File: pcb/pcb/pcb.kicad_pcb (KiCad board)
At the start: 2 copper layers, 40 x 47 mm, 8 parts, among them SW1 SW_SPDT, U1 Pimoroni_LiPo_Amigo, U2 Timecube_Accelerometer, U3 Tiny2040, U5 E-ink_Driver

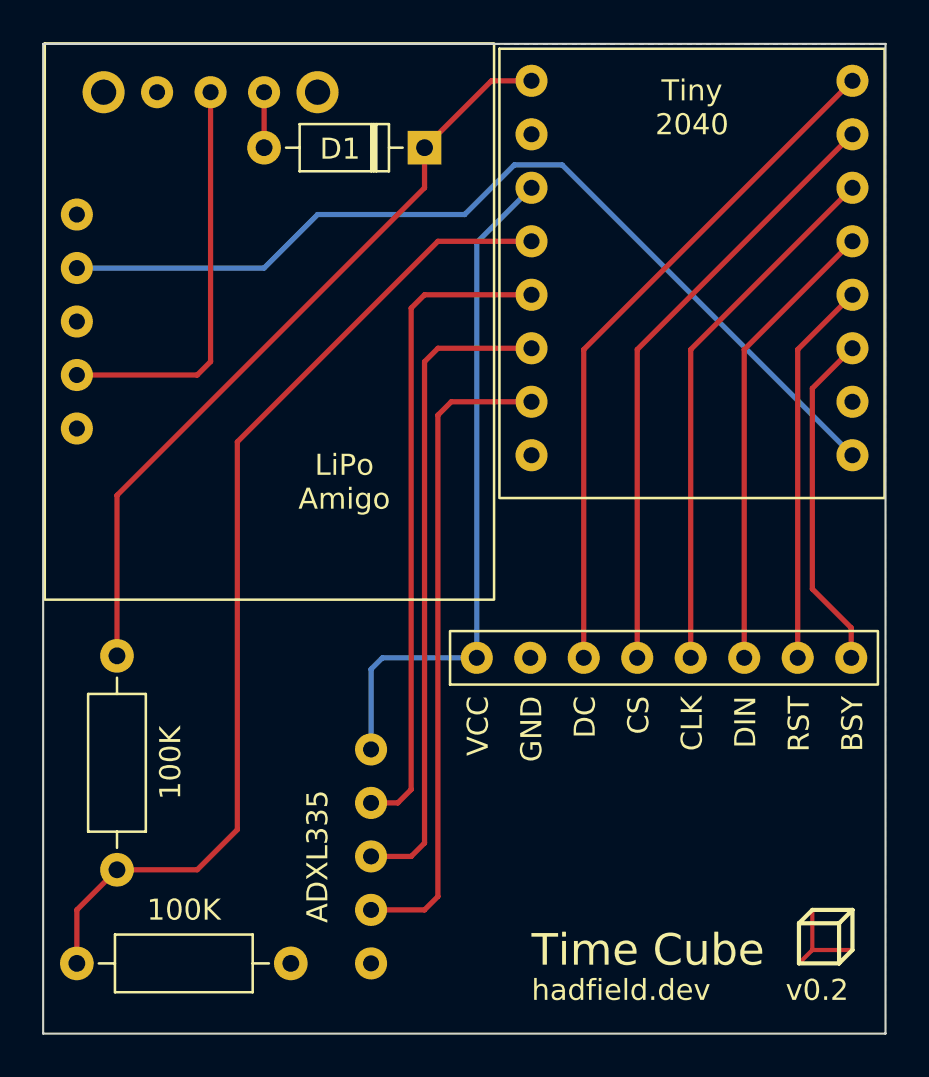
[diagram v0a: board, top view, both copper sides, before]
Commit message: pcb 0.3, inner v4, flash_files update
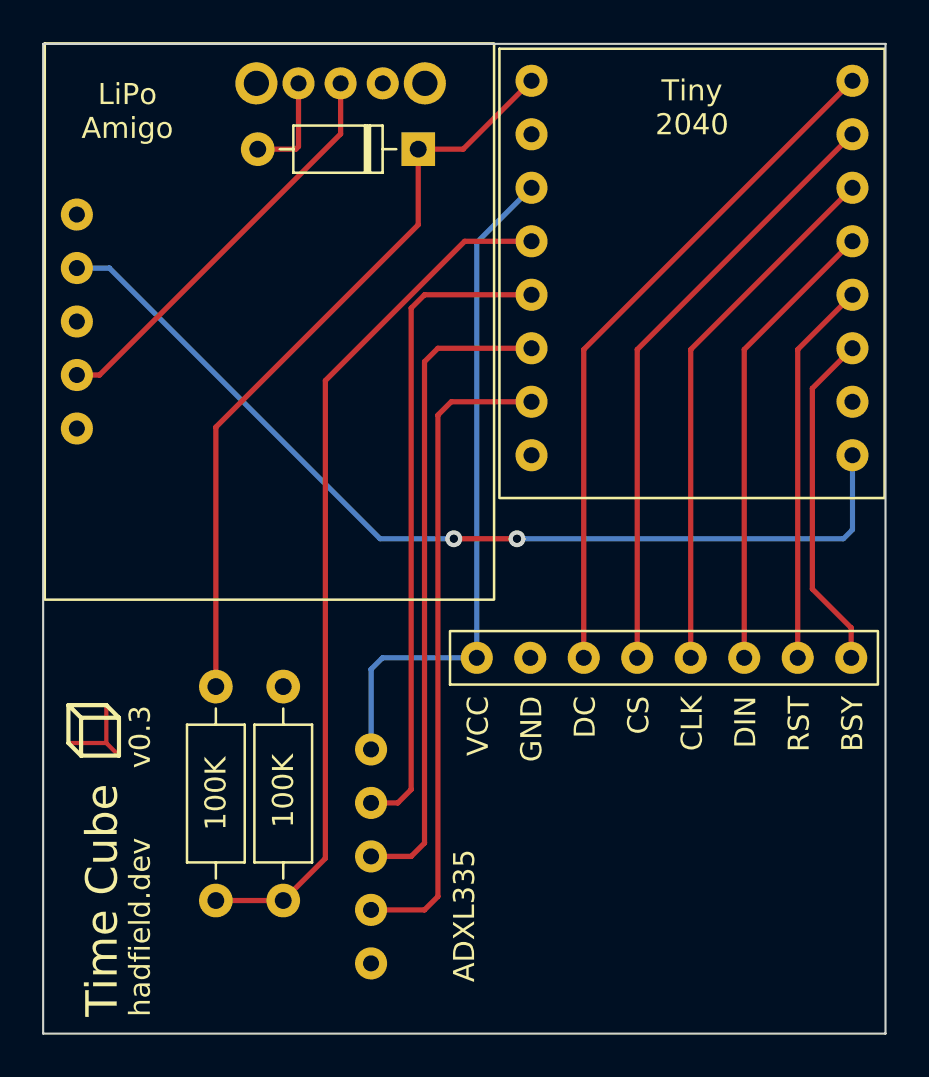
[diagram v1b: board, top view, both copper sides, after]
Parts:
- SW1: moved to F.Cu
- moved SW1 11.7 mm to (101.1, 86.9)
- moved R2 10.2 mm to (111.4, 110.7), turned to 90 degrees
- moved R1 4.92 mm to (108.2, 100.5)
- moved D1 0.31 mm to (117.8, 75.0)
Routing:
- net Net-(R1-Pad2): track 48.1 -> 41.2 mm
- net Net-(SW1-Pad3): track 2.64 -> 4.99 mm
- net Net-(U3-Pad9): track 44.6 -> 45.9 mm, vias 0 -> 2
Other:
- board text added: "v0.3"
- board text removed: "v0.2"
